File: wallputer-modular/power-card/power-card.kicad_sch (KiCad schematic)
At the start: 134 parts, among them J2 Power, Q1 FQP27P06, Q2 IRLZ44N, SW1 reset, U1 TLC555CD, U12 74HC04, U16 74HC04, U17 74HC04, U18 74HC04, U2 74HC04, U3 74HC04

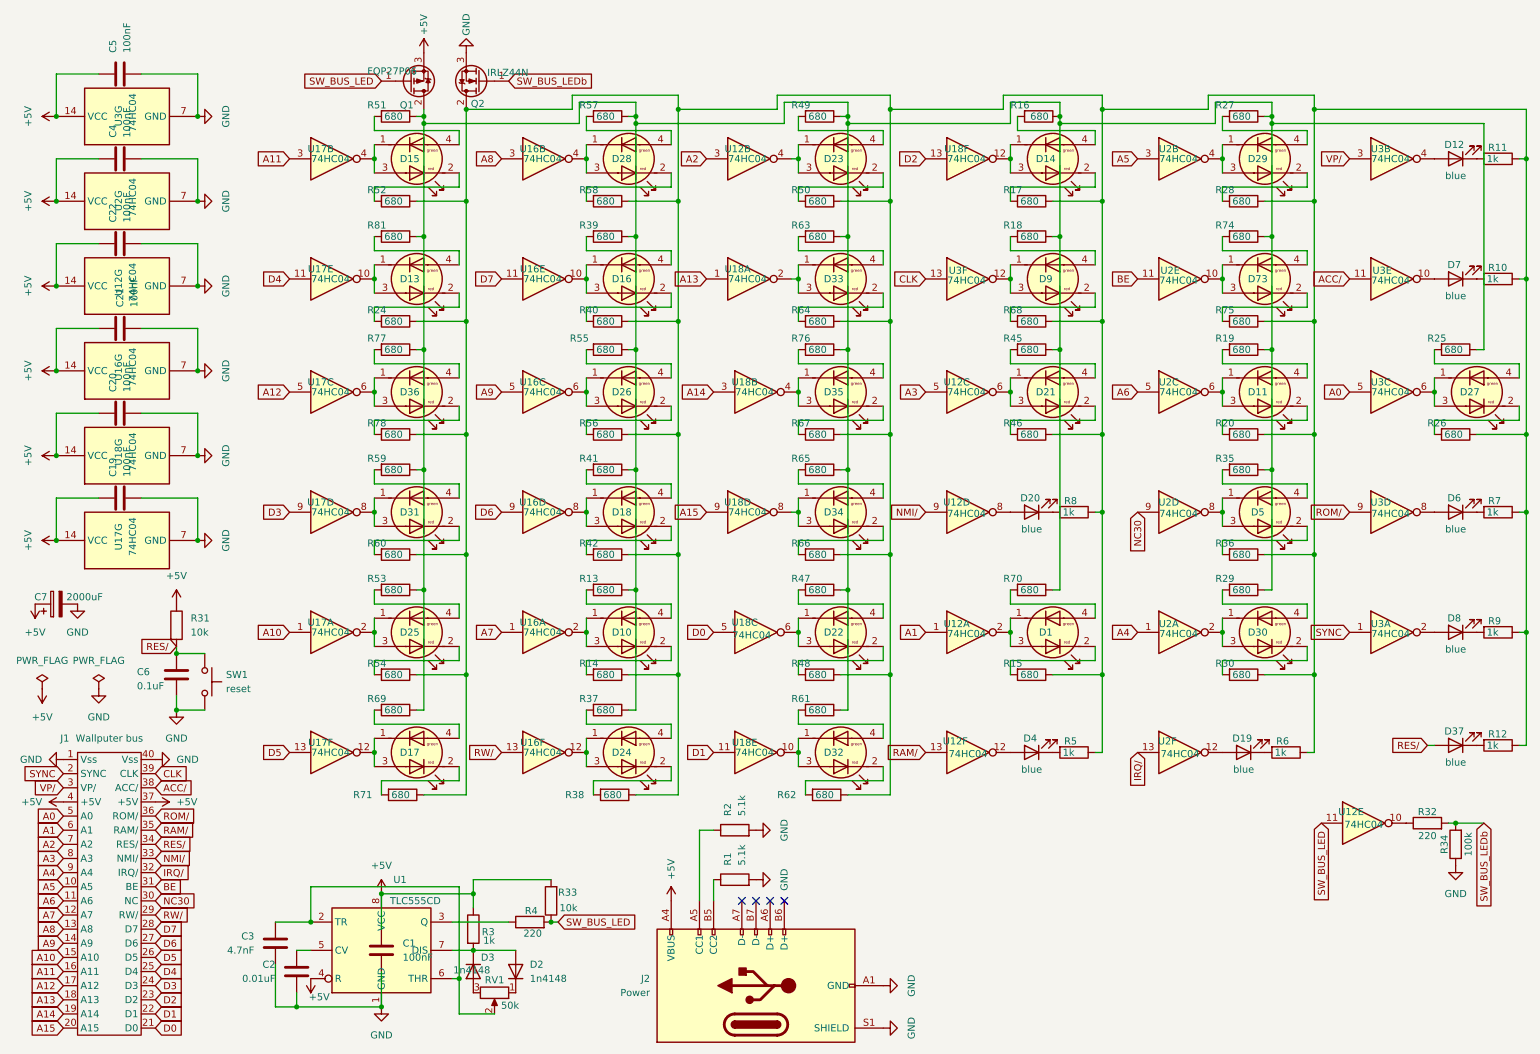
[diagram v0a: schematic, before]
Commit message: begin wiring memory card
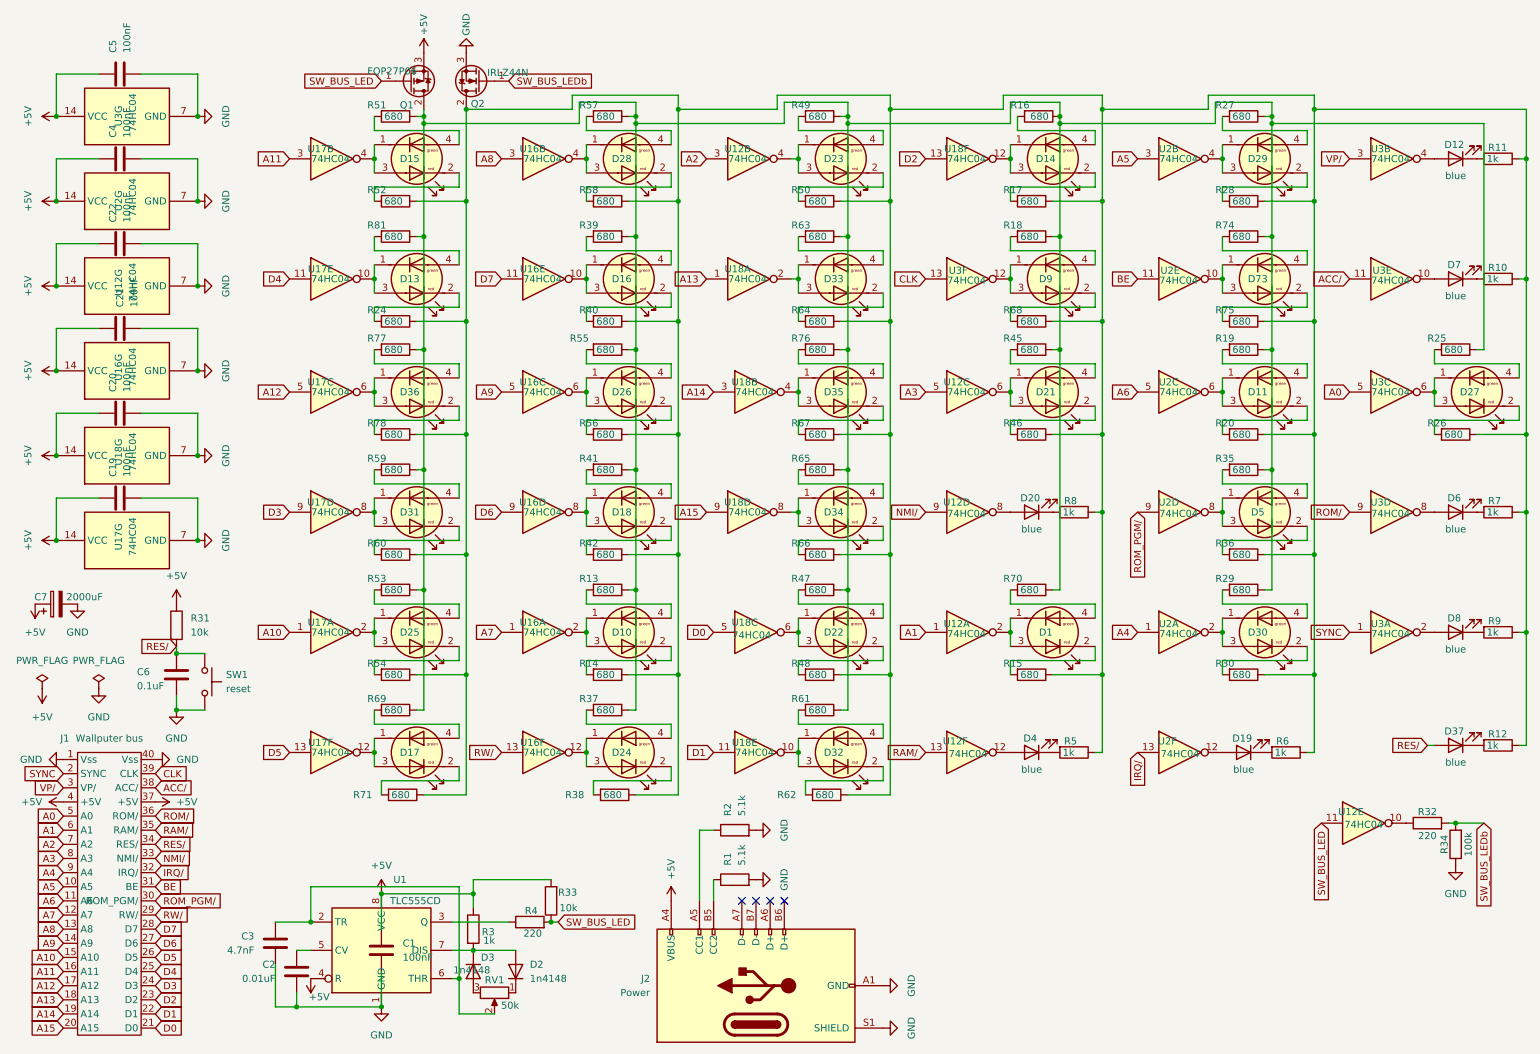
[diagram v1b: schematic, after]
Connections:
- net NC30 renamed ROM_PGM/
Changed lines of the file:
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@@
 		)
 	)
-	(global_label "NC30"
+	(global_label "ROM_PGM{slash}"
 		(shape input)
 		(at 36.83 171.45 0)
@@
 		)
 	)
-	(global_label "NC30"
+	(global_label "ROM_PGM{slash}"
 		(shape input)
 		(at 213.36 101.6 270)
